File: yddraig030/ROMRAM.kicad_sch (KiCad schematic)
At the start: 10 parts, among them U401 SST39SF040, U402 AS6C4008-55PCN, U403 SST39SF040, U404 AS6C4008-55PCN, U405 74LS32

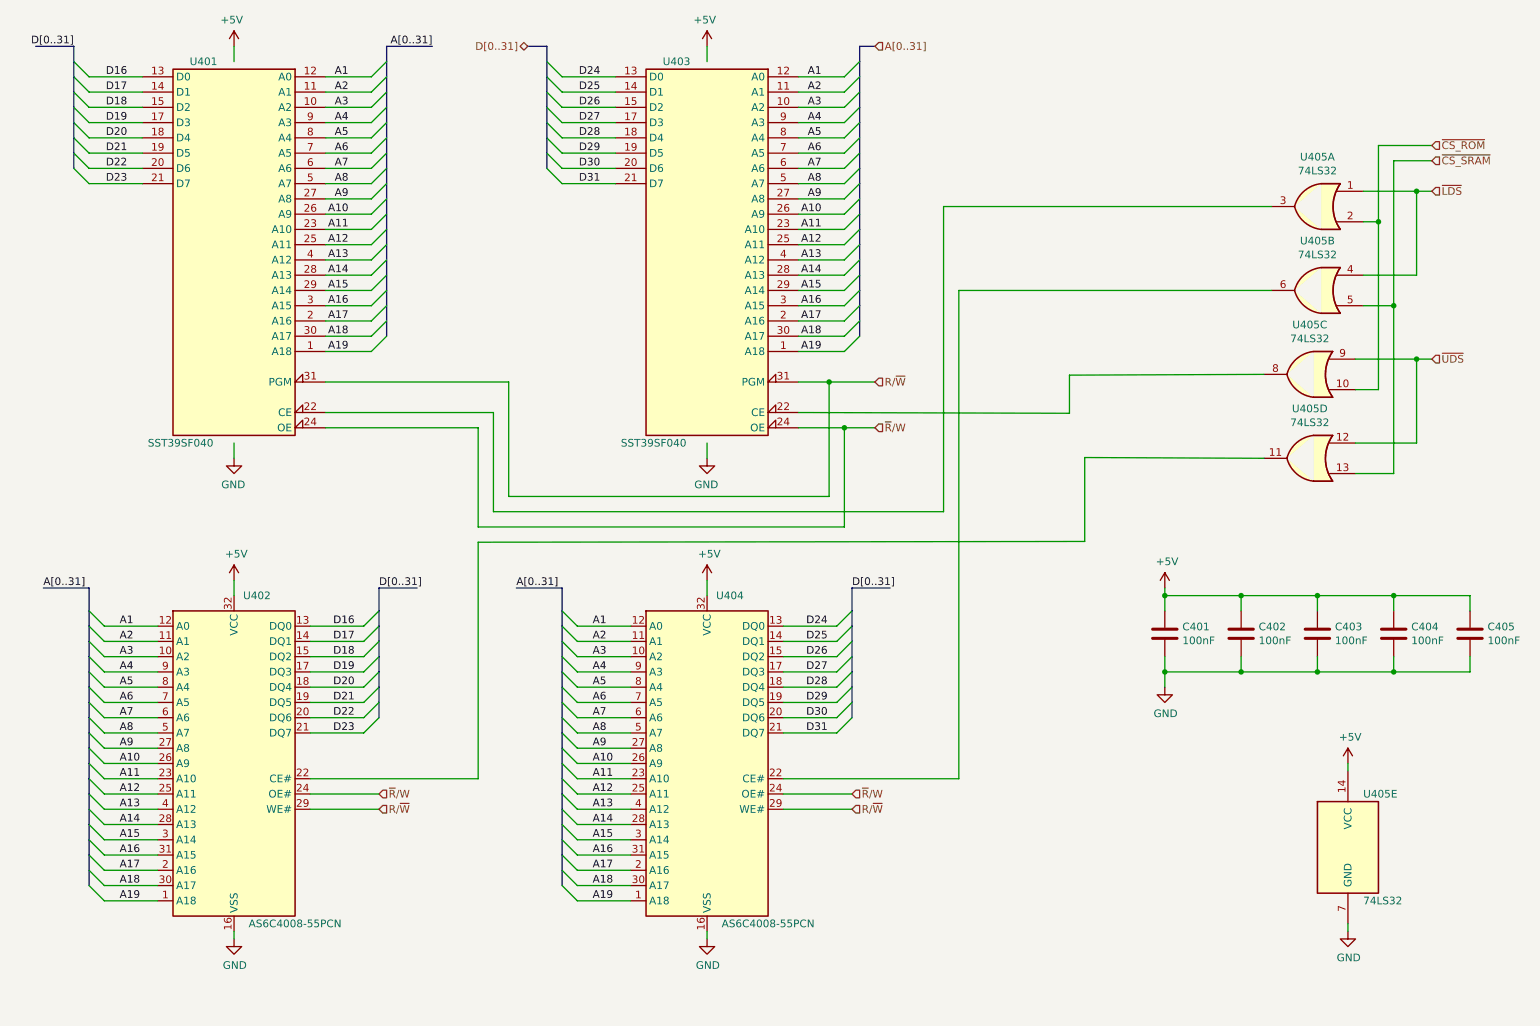
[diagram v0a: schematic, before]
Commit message: More changes in yddraig030 layout
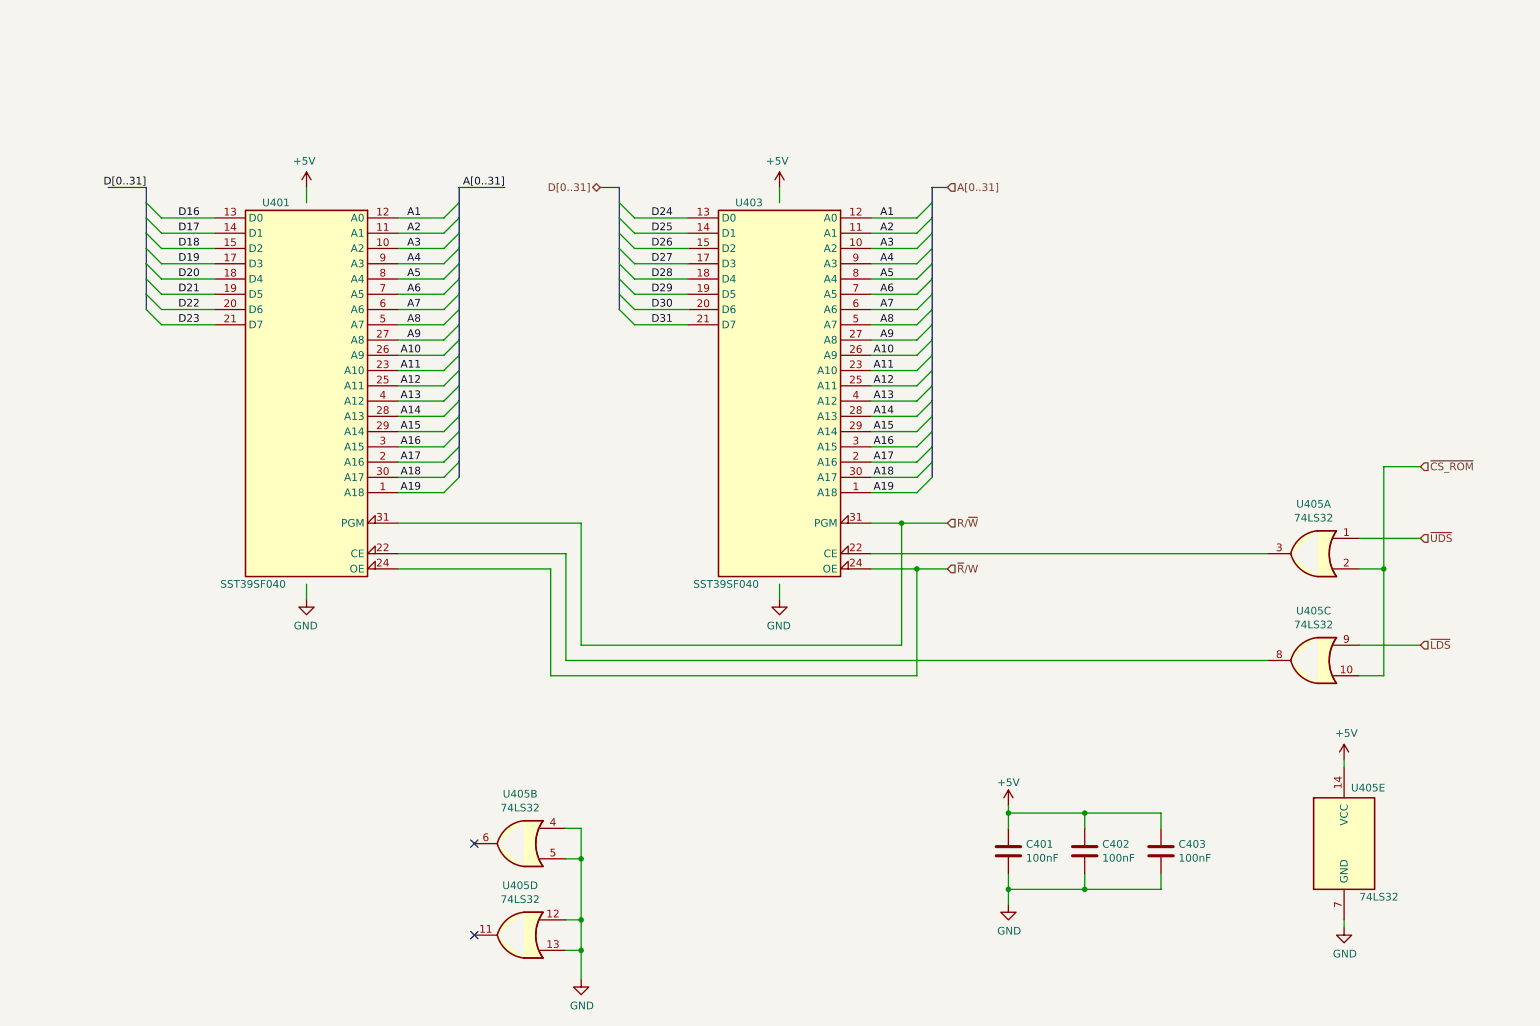
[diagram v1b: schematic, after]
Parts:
- removed C404, C405: 100nF, Capacitor_THT:C_Disc_D3.8mm_W2.6mm_P2.50mm, symbol Device:C
- removed U402, U404: AS6C4008-55PCN, Package_DIP:DIP-32_W15.24mm, symbol Memory_RAM:AS6C4008-55PCN
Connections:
- net ~{CS_SRAM} is gone; now on net GND: U405.13, U405.5
- net GND: now also U405.12, U405.4
- net ~{LDS}: now also U405.9; no longer U405.1, U405.4
- net ~{UDS}: now also U405.1; no longer U405.12, U405.9
- net at U401.22 (CE): now also U405.8; no longer U405.3
- net at U403.22 (CE): now also U405.3; no longer U405.8
- no-connect marks 0 -> 2
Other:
- moved on the sheet: C401, C402, C403, U401, U403, U405A, U405B, U405C, U405D, U405E
